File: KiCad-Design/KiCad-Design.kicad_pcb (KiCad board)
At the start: 2 copper layers, 35 x 35 mm, 68 parts, among them J1 USB_B_Micro, J2 Battery, J3 Ext, J4 OLED, Q1 SI2301, Q2 SI2301, Q3 SI2307CDS-T1-GE3, SW1 MCU BLE Adv, SW2 MCU FLASH, SW3 MCU RESET, U1 PMBT3904, U2 BME280, U3 CP2104, U4 LTC4054ES5-4.2, U5 PMBT3904, U6 PMBT3904, U7 BME680, U8 AP2112K-3.3, U9 ttgo-32-micro-symbols

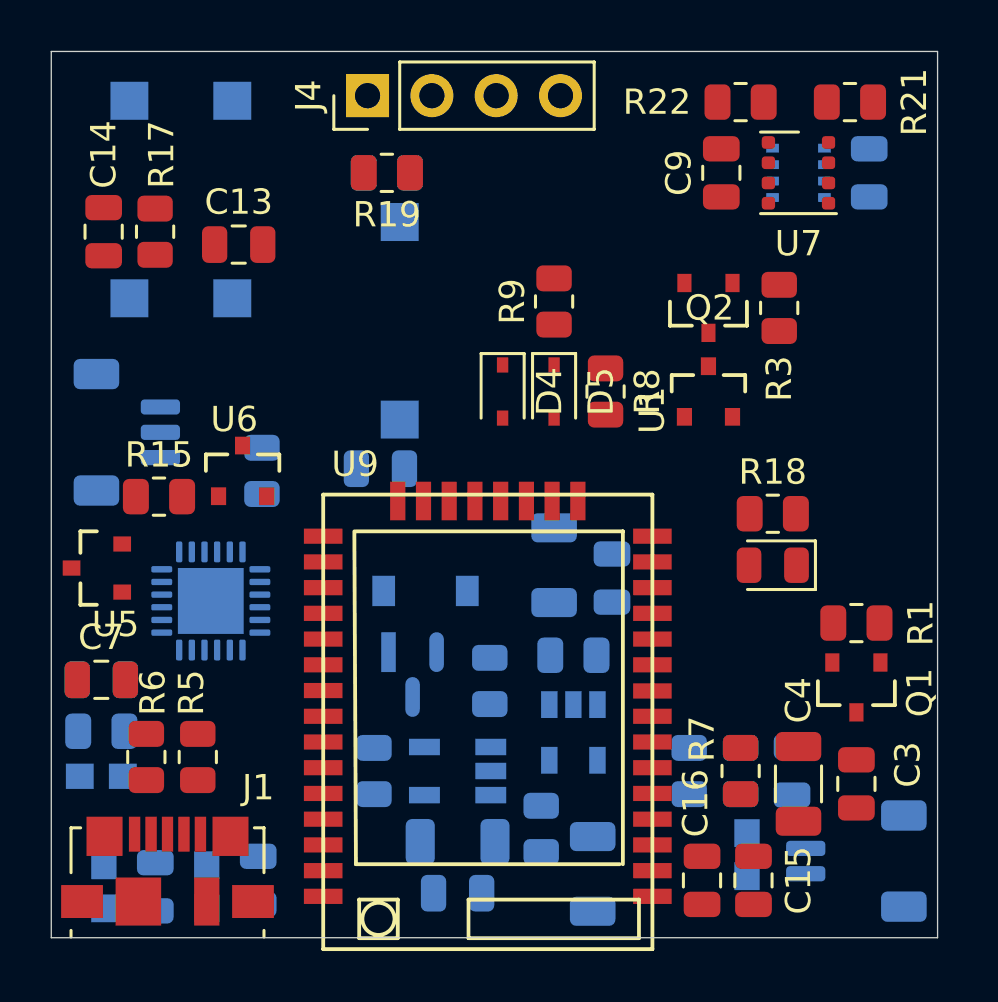
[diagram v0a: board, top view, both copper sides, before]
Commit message: PCB : Initial PCB Design
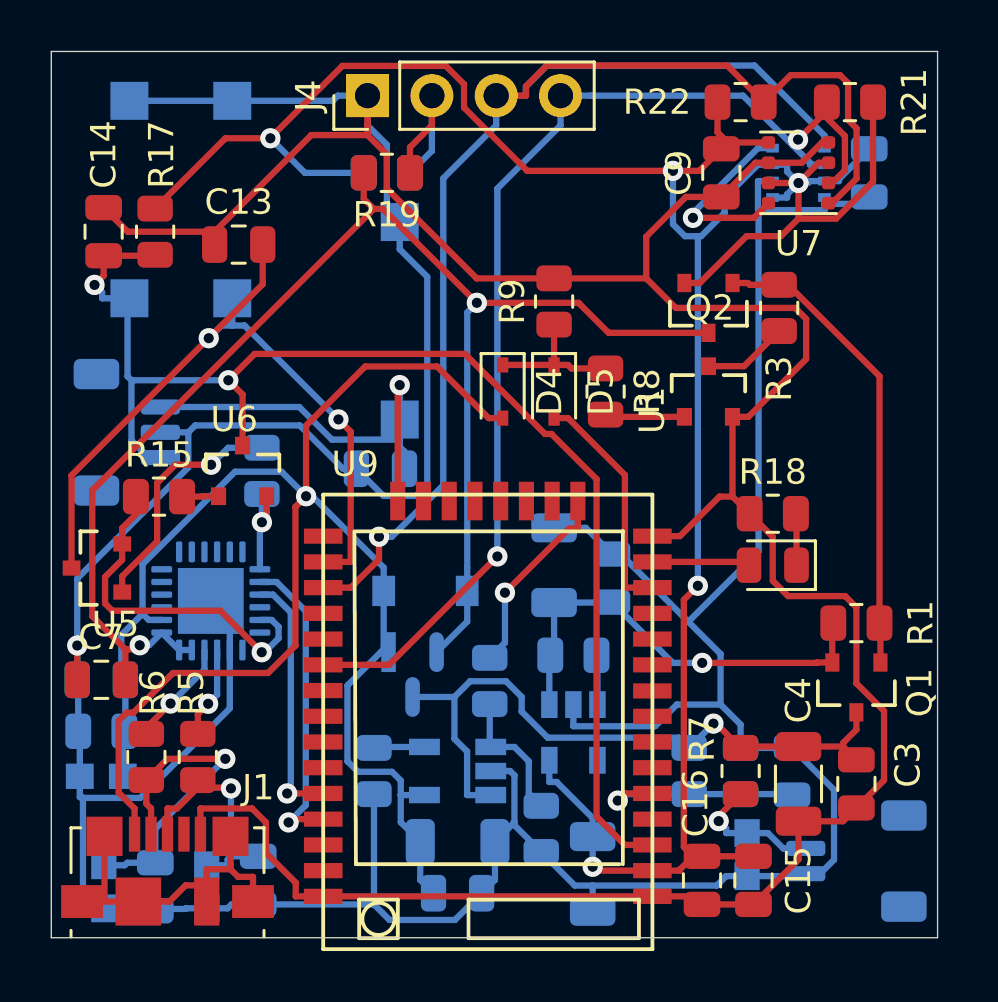
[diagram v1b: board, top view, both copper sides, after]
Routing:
- net GND: track 0.00 -> 271.9 mm, vias 0 -> 1
- net +3V3: track 0.00 -> 102.3 mm, vias 0 -> 5
- net +5V: track 0.00 -> 70.6 mm, vias 0 -> 1
- net MCU_SCL: track 0.00 -> 59.7 mm, vias 0 -> 1
- net +VSW: track 0.00 -> 58.2 mm, vias 0 -> 2
- net MCU_RESET: track 0.00 -> 51.8 mm, vias 0 -> 2
- net MCU_SDA: track 0.00 -> 45.2 mm, vias 0 -> 2
- net MCU_FLASH: track 0.00 -> 30.8 mm, vias 0 -> 2
- net +BATT: track 0.00 -> 26.8 mm, vias 0 -> 1
- net Net-(Q1-Pad1): track 0.00 -> 18.7 mm
- net MCU_BLE_Adv: track 0.00 -> 18.0 mm, vias 0 -> 1
- net VCC: track 0.00 -> 17.7 mm, vias 0 -> 1
- net Net-(R15-Pad1): track 0.00 -> 13.9 mm, vias 0 -> 1
- net Net-(J1-Pad6): track 0.00 -> 13.3 mm
- net Net-(C2-Pad2): track 0.00 -> 13.0 mm, vias 0 -> 1
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
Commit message: PCB : Finalizing the PCB v1
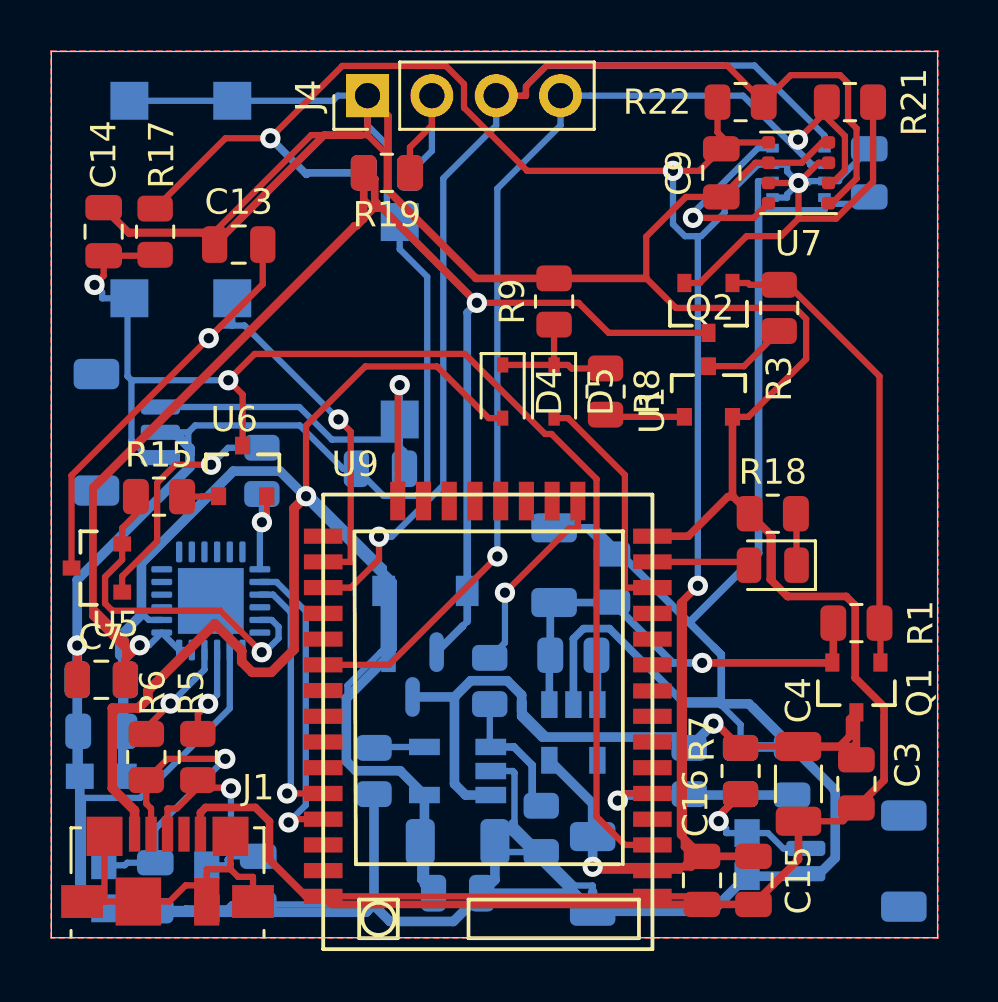
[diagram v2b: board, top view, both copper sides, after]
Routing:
- net GND: track 271.9 -> 398.5 mm
- net +VSW: track 58.2 -> 105.6 mm
- net +5V: track 70.6 -> 114.2 mm
- net +3V3: track 102.3 -> 123.6 mm
- net +BATT: track 26.8 -> 46.8 mm
- net MCU_BAT_REF: track 8.49 -> 15.5 mm
- added copper zone on B.Cu, net GND
- added copper zone on F.Cu, net GND
